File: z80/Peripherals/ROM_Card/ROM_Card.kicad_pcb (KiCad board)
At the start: 2 copper layers, 24 x 17.3 mm, 14 parts, among them J1 Conn_02x20_Top_Bottom, SW1 SW_SPDT, SW10 SW_SPDT, SW2 SW_SPDT, SW3 SW_SPDT, SW4 SW_SPDT, SW5 SW_SPDT, SW6 SW_SPDT, SW7 SW_SPDT, SW8 SW_SPDT, SW9 SW_SPDT, U1 74HC244, U2 SST39SF040, U5 74AHC1G02

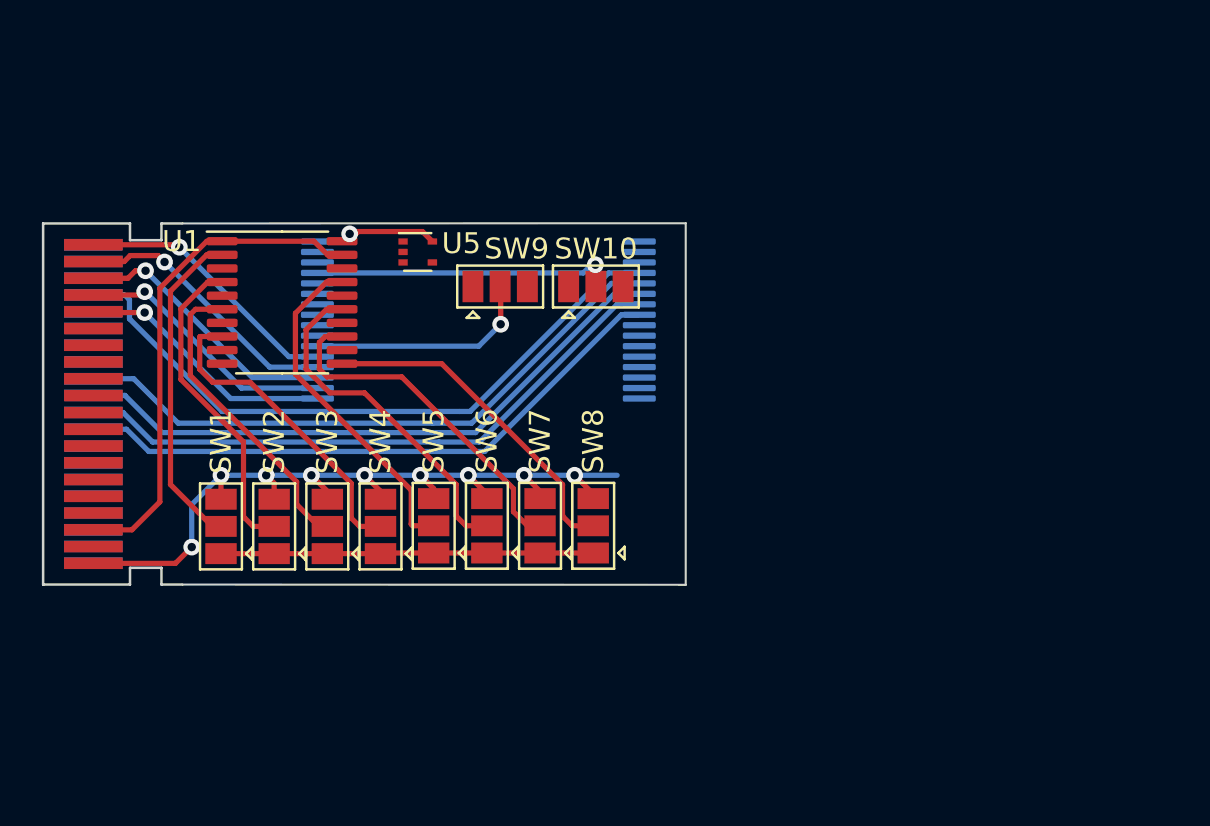
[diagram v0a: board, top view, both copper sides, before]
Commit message: finished v2 of hardware, updated eeprom prog pins
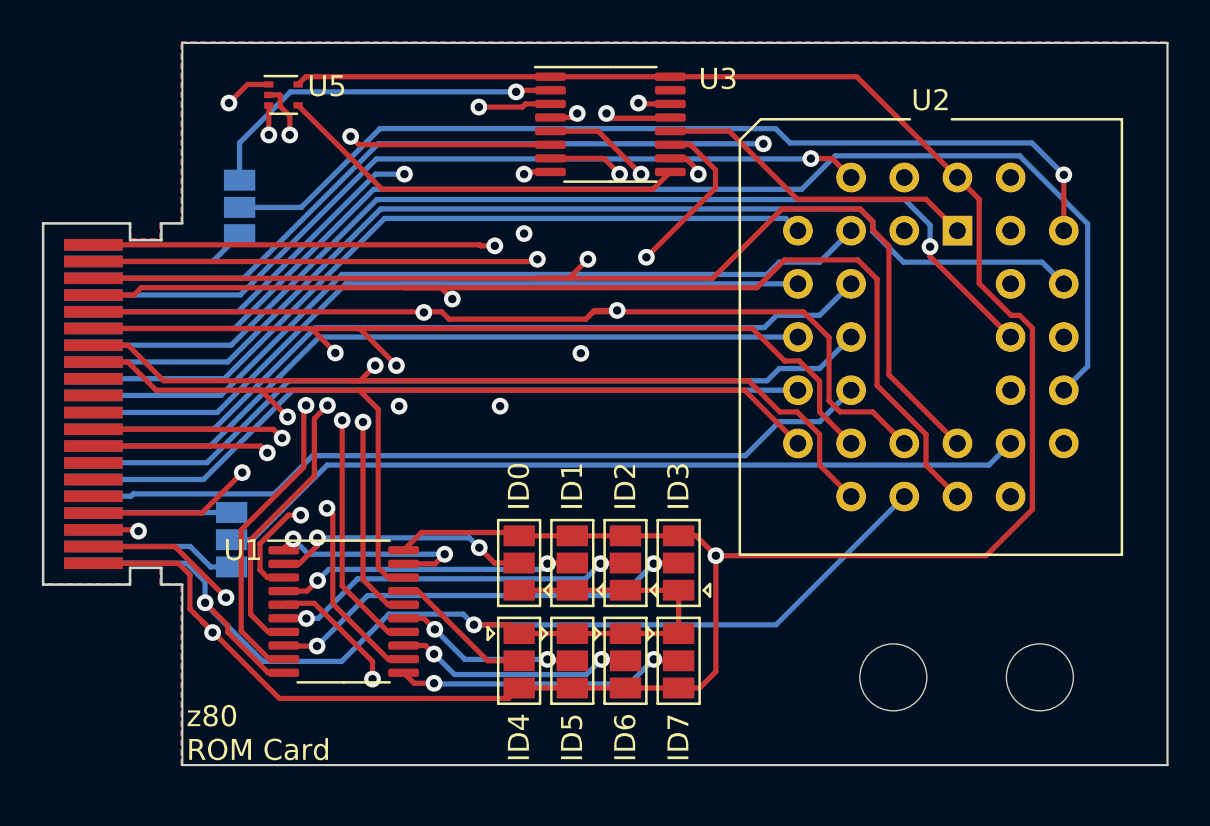
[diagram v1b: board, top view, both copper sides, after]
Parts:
- added REF**: MountingHole_3.2mm_M3, MountingHole:MountingHole_3.2mm_M3, F.Cu at (170.3, 118.6)
- added REF**: MountingHole_3.2mm_M3, MountingHole:MountingHole_3.2mm_M3, F.Cu at (177.3, 118.6)
- added U3: 74LS174, Package_SO:TSSOP-16_4.4x5mm_P0.65mm, F.Cu at (156.8, 92.2)
- SA14: renamed from SW10; moved to B.Cu
- SCS1: renamed from SW9; moved to B.Cu
- U2: footprint Package_SO:TSOP-I-32_14.4x8mm_P0.5mm -> Package_LCC:PLCC-32_THT-Socket; moved to F.Cu
- moved U2 23.3 mm to (173.4, 97.3), turned to 0 degrees
- moved SCS1 17.6 mm to (138.7, 112.0), turned to 90 degrees
- moved SA14 17.4 mm to (139.1, 96.2), turned to -90 degrees
- moved U1 15.1 mm to (144.0, 115.5)
- moved ID0 14.3 mm to (152.4, 113.2)
- moved ID3 14.3 mm to (160.0, 113.2)
- moved ID1 14.3 mm to (155.0, 113.2)
- moved ID2 14.3 mm to (157.5, 113.2)
- moved U5 9.87 mm to (141.2, 90.8)
- moved ID7 7.63 mm to (160.0, 117.8), turned to -90 degrees
- moved ID4 7.63 mm to (152.4, 117.8), turned to -90 degrees
- moved ID5 7.63 mm to (155.0, 117.8), turned to -90 degrees
- moved ID6 7.63 mm to (157.5, 117.8), turned to -90 degrees
- renumbered SW1 to ID0, SW2 to ID1, SW3 to ID2, SW4 to ID3, SW5 to ID4, SW6 to ID5, SW7 to ID6, SW8 to ID7
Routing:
- net +5V: track 45.9 -> 148.5 mm, vias 10 -> 2
- net GND: track 17.8 -> 109.9 mm, vias 0 -> 4
- net /D5: track 13.0 -> 94.4 mm, vias 1 -> 4
- net /D2: track 0.00 -> 79.4 mm, vias 0 -> 4
- net /D4: track 12.7 -> 88.3 mm, vias 1 -> 4
- net /D0: track 0.00 -> 74.2 mm, vias 0 -> 2
- net /D1: track 0.00 -> 74.1 mm, vias 0 -> 4
- net /D7: track 12.9 -> 82.6 mm, vias 1 -> 2
- net /D3: track 12.4 -> 76.6 mm, vias 1 -> 4
- net /D6: track 13.0 -> 76.3 mm, vias 1 -> 2
- net /A10: track 0.00 -> 60.7 mm
- net /A11: track 0.00 -> 52.3 mm, vias 0 -> 1
- net /PGM/5V: track 0.00 -> 52.1 mm, vias 0 -> 1
- net /A8: track 0.00 -> 51.1 mm
- net /A9: track 0.00 -> 50.3 mm, vias 0 -> 1
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- added copper zone on B.Cu, net GND
- added copper zone on F.Cu, net GND
- added copper zone on In1.Cu, net GND
- added copper zone on In2.Cu, net GND
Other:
- board size 24 x 17.3 mm -> 47.1 x 34.5 mm
- copper layers 2 -> 4
- board text added: "z80 ROM Card"
